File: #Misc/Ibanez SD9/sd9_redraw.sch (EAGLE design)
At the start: 73 parts, among them IC101 RC4558, Q101 2SC1815BL, Q102 1SK44SP, Q103 2SC1815BL, Q104 2SK44SP, Q105 2SC1815BL, Q106 2SC1815BL, Q107 2SC1815BL

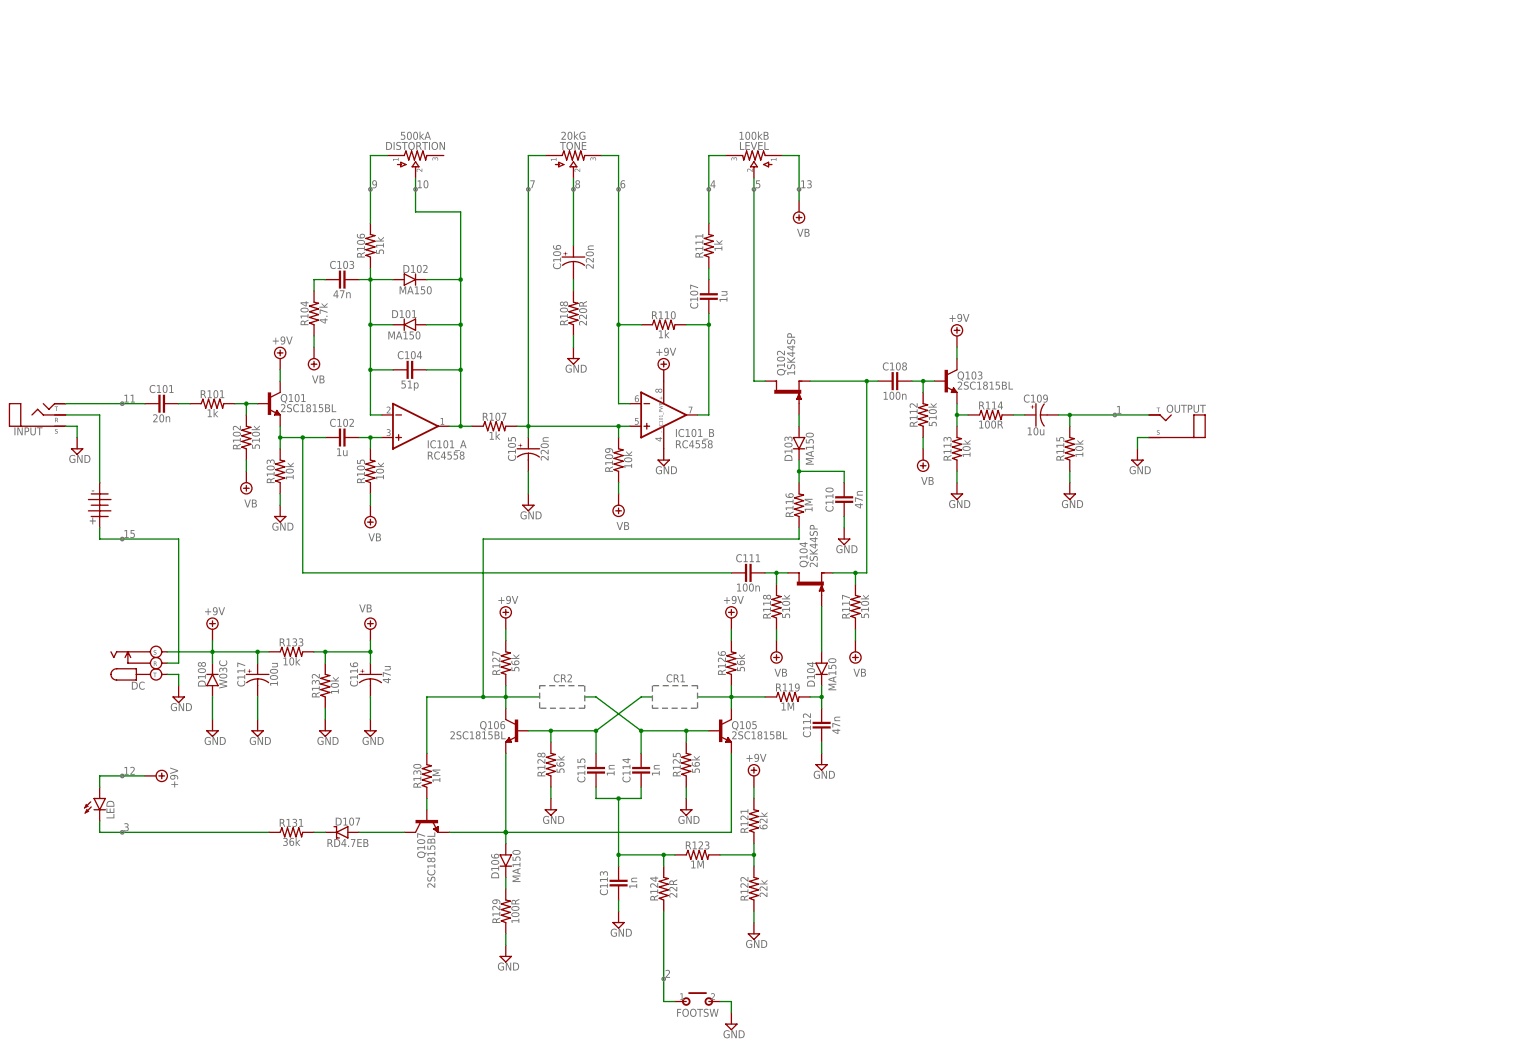
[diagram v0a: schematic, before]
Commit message: 20200325/10:41
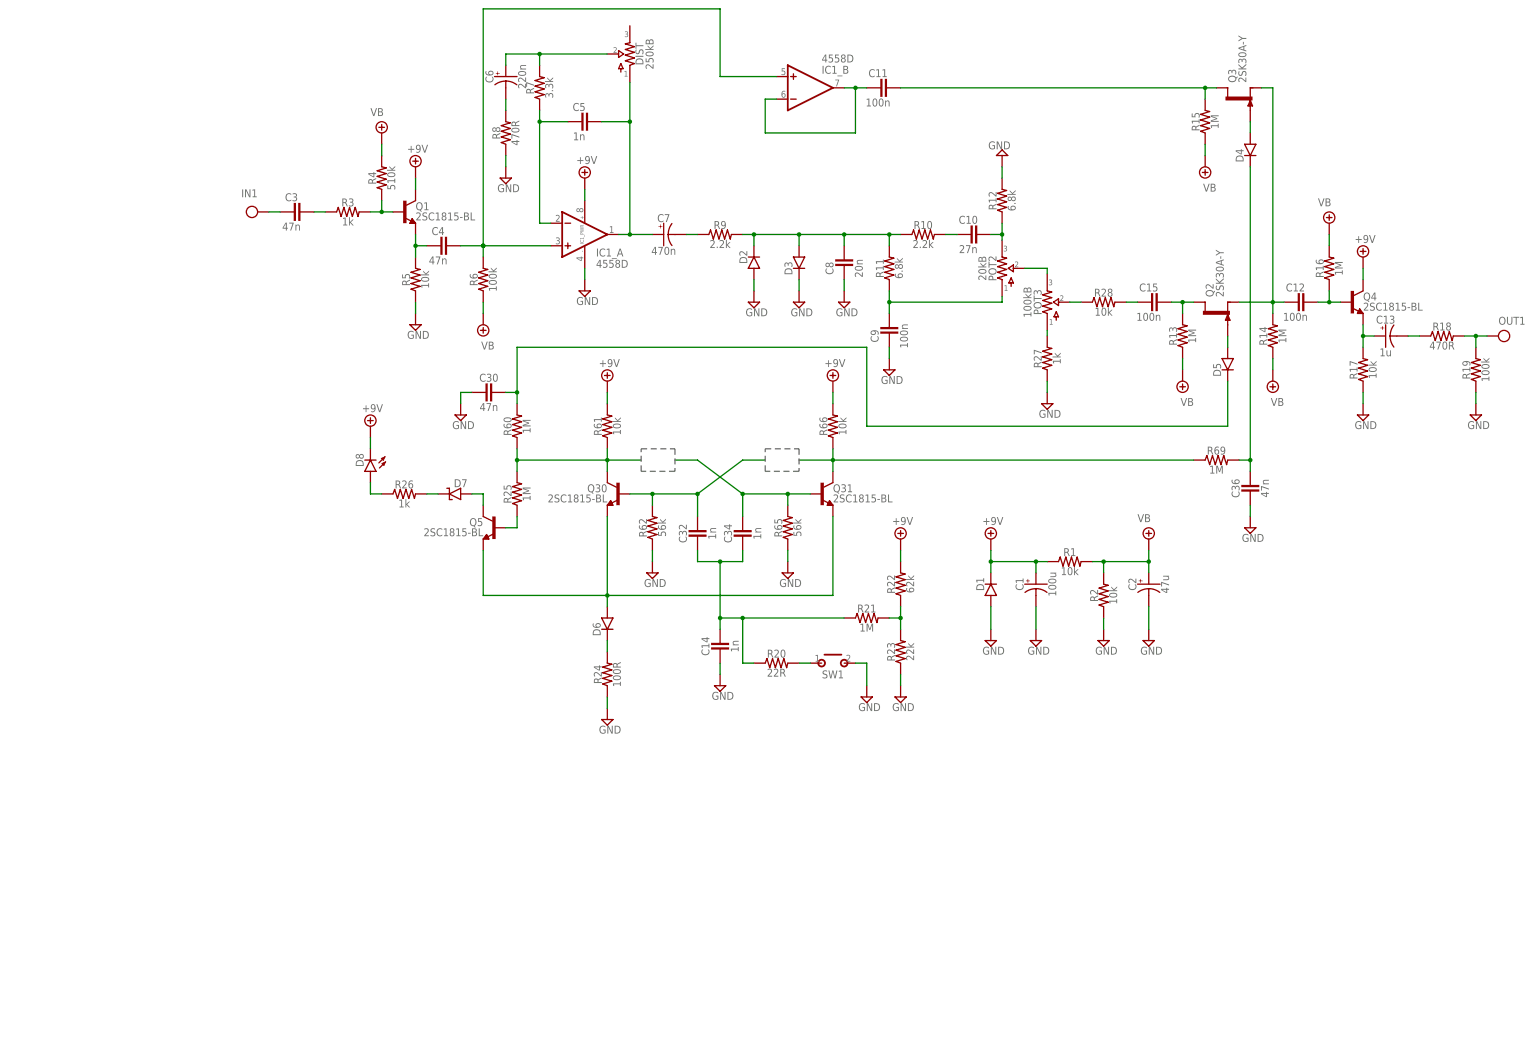
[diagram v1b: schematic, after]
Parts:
- removed BATTERY: BATTERY, pedals-jacks:BATTERY
- removed C101: 20n, pedals-capacitors-film:CER/FILMBOX.1
- removed C102, C107: 1u, pedals-capacitors-film:CER/FILMBOX.1
- removed C103, C110, C112: 47n, pedals-capacitors-film:CER/FILMBOX.1
- removed C104: 51p, pedals-capacitors-film:CER/FILMBOX.1
- removed C105, C106: 220n, pedals-capacitors-elec:0500
- removed C108, C111: 100n, pedals-capacitors-film:CER/FILMBOX.1
- removed C109: 10u, pedals-capacitors-elec:0500
- removed C113, C114, C115: 1n, pedals-capacitors-film:CER/FILMBOX.1
- removed C116: 47u, pedals-capacitors-elec:0500
- removed C117: 100u, pedals-capacitors-elec:0500
- removed D101, D102, D103, D104, D106: MA150, pedals-diodes:DO35.2
- removed D107: RD4.7EB, pedals-diodes:ZENER.2
- removed D108: W03C, pedals-diodes:DO35.2
- removed DC: DCJACK, pedals-jacks:DC_KOBICONN
- removed DISTORTION: 500kA, pedals-potentiometers:POTS16MM
- removed FOOTSW: MOMENTARY, pedals-switches:MOMENTARY
- removed IC101: RC4558, pedals-integrated circuits:DUALTH
- removed INPUT: (no value), pedals-jacks:STEREO3PADS
- removed LED: LED, pedals-diodes:LED
- removed LEVEL: 100kB, pedals-potentiometers:POTS16MM
- removed OUTPUT: (no value), pedals-jacks:MONO
- removed Q101, Q103: 2SC1815BL, pedals-transistors:2N3904
- removed Q102: 1SK44SP, pedals-transistors:2N5457
- removed Q104: 2SK44SP, pedals-transistors:2N5457
- removed Q105, Q106, Q107: 2SC1815BL, pedals-transistors:2SC828A
- removed R101, R107, R110, R111: 1k, pedals-resistors:R_.3B
- removed R102, R112, R117, R118: 510k, pedals-resistors:R_.3B
- removed R103, R105, R109, R113, R115, R132, R133: 10k, pedals-resistors:R_.3B
- removed R104: 4.7k, pedals-resistors:R_.3B
- removed R106: 51k, pedals-resistors:R_.3B
- removed R108: 220R, pedals-resistors:R_.3B
- removed R114, R129: 100R, pedals-resistors:R_.3B
- removed R116, R119, R123, R130: 1M, pedals-resistors:R_.3B
- removed R121: 62k, pedals-resistors:R_.3B
- removed R122: 22k, pedals-resistors:R_.3B
- removed R124: 22R, pedals-resistors:R_.3B
- removed R125, R126, R127, R128: 56k, pedals-resistors:R_.3B
- removed R131: 36k, pedals-resistors:R_.3B
- removed TONE: 20kG, pedals-potentiometers:POTS16MM
- added C1: 100u, pedals-capacitors-elec:0500
- added C10: 27n, pedals-capacitors-film:CER/FILMBOX.1
- added C11, C12, C15, C9: 100n, pedals-capacitors-film:CER/FILMBOX.1
- added C13: 1u, pedals-capacitors-elec:0500
- added C14, C32, C34, C5: 1n, pedals-capacitors-film:CER/FILMBOX.1
- added C2: 47u, pedals-capacitors-elec:0500
- added C3, C30, C36, C4: 47n, pedals-capacitors-film:CER/FILMBOX.1
- added C6: 220n, pedals-capacitors-elec:0500
- added C7: 470n, pedals-capacitors-elec:0500
- added C8: 20n, pedals-capacitors-film:CER/FILMBOX.1
- added D1, D2, D3, D4, D5, D6: (no value), pedals-diodes:DO41.2
- added D7: (no value), pedals-diodes:ZENER.2
- added D8: LED, pedals-diodes:LED
- added DIST: 250kB, pedals-potentiometers:POTS16MM
- added IC1: 4558D, pedals-integrated circuits:DUALTH
- added POT2: 20kB, pedals-potentiometers:POTS16MM
- added POT3: 100kB, pedals-potentiometers:POTS16MM
- added Q1, Q4: 2SC1815-BL, pedals-transistors:2N3904
- added Q2, Q3: 2SK30A-Y, pedals-transistors:2SK170
- added Q30, Q31, Q5: 2SC1815-BL, pedals-transistors:2SC828A
- added R1, R17, R2, R28, R5, R61, R66: 10k, pedals-resistors:R_.3B
- added R10, R9: 2.2k, pedals-resistors:R_.3B
- added R11, R12: 6.8k, pedals-resistors:R_.3B
- added R13, R14, R15, R16, R21, R25, R60, R69: 1M, pedals-resistors:R_.3B
- added R18, R8: 470R, pedals-resistors:R_.3B
- added R19, R6: 100k, pedals-resistors:R_.3B
- added R20: 22R, pedals-resistors:R_.3B
- added R22: 62k, pedals-resistors:R_.3B
- added R23: 22k, pedals-resistors:R_.3B
- added R24: 100R, pedals-resistors:R_.3B
- added R26, R27, R3: 1k, pedals-resistors:R_.3B
- added R4: 510k, pedals-resistors:R_.3B
- added R62, R65: 56k, pedals-resistors:R_.3B
- added R7: 3.3k, pedals-resistors:R_.3B
- added SW1: MOMENTARY, pedals-switches:MOMENTARY
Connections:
- removed net N$1: C101.2, INPUT.T
- removed net N$23: C108.1, Q103.B, R112.2
- removed net N$42: D107.A, Q107.C
- new net IN: C3.2
- new net N$62: C36.1, D4.C, R69.2
- new net N$72: C30.1, D5.C, R60.2
- new net OUT: R18.2, R19.2
- net +9V: now also C1.+, D1.C, D8.C, IC1_PWR.V+, Q1.C, Q4.C, R1.1, R22.2, R61.2, R66.2; no longer C117.+, D108.C, DC.S, IC101_PWR.V+, LED.A, Q101.C, Q103.C, R121.2, R126.2, R127.2, R133.1
- net GND: now also C1.-, C14.2, C2.-, C30.2, C36.2, C8.2, C9.2, D1.A, D2.A, D3.C, IC1_PWR.V-, R12.2, R17.1, R19.1, R2.1, R23.1, R24.1, R27.1, R5.1, R62.1, R65.1, R8.1, SW1.S; no longer C105.-, C110.2, C112.2, C113.2, C116.-, C117.-, D108.A, DC.T, FOOTSW.S, IC101_PWR.V-, INPUT.S, OUTPUT.SLEEVE, R103.1, R108.1, R113.1, R115.1, R122.1, R125.1, R128.1, R129.1, R132.1
- net N$10: now also C7.-, R9.1; no longer C105.+, IC101_B.+IN, R107.2, R109.2, TONE.1
- net N$11: now also C8.1, D2.C, D3.A, R10.1, R11.2, R9.2; no longer IC101_B.-IN, R110.1, TONE.3
- net N$12: now also POT2.2, POT3.3; no longer C107.2, IC101_B.OUT, R110.2
- net N$13: now also C10.2, R10.2; no longer C107.1, R111.1
- net N$14: now also C10.1, POT2.3, R12.1; no longer C106.+, TONE.2
- net N$15: now also C9.1, POT2.1, R11.1; no longer C106.-, R108.2
- net N$16: now also C11.2, IC1_B.-IN, IC1_B.OUT; no longer LEVEL.3, R111.2
- net N$17: now also C11.1, Q3.D, R15.2; no longer LEVEL.2, Q102.D
- net N$18: now also C12.1, Q4.B, R16.1; no longer C108.2, Q102.S, Q104.S, R117.2
- net N$19: now also C12.2, Q2.S, Q3.S, R14.2; no longer D103.A, Q102.G
- net N$2: now also C3.1, R3.1; no longer BATTERY.P$2, INPUT.R
- net N$20: now also C15.1, Q2.D, R13.2; no longer C110.1, D103.C, R116.2
- net N$21: now also C13.+, Q4.E, R17.2; no longer D104.A, Q104.G
- net N$22: now also C13.-, R18.1; no longer C112.1, D104.C, R119.2
- net N$24: now also R20.2, SW1.P; no longer Q103.E, R113.2, R114.1
- net N$25: now also D4.A, Q3.G; no longer C109.+, R114.2
- net N$26: now also D5.A, Q2.G; no longer C109.-, OUTPUT.TIP, R115.2
- net N$27: now also D6.A, Q30.E, Q31.E, Q5.E; no longer C111.1, Q104.D, R118.2
- net N$28: now also Q30.C, R25.2, R60.1, R61.1; no longer BATTERY.P$1, DC.R
- net N$29: now also Q5.B, R25.1; no longer Q106.C, R116.1, R127.1, R130.2
- net N$3: now also Q1.B, R3.2, R4.1; no longer Q101.B, R101.2, R102.2
- net N$30: now also D7.A, Q5.C; no longer Q107.B, R130.1
- net N$31: now also Q31.C, R66.1, R69.1; no longer Q105.C, R119.1, R126.1
- net N$32: now also C32.1, Q30.B, R62.2; no longer C115.1, Q106.B, R128.2
- net N$33: now also D7.C, R26.2; no longer C101.1, R101.1
- net N$34: now also C34.1, Q31.B, R65.2; no longer C114.1, Q105.B, R125.2
- net N$35: now also C14.1, C32.2, C34.2, R20.1, R21.1; no longer D106.A, Q105.E, Q106.E, Q107.E
- net N$36: now also D8.A, R26.1; no longer C113.1, C114.2, C115.2, R123.1, R124.2
- net N$37: now also D6.C, R24.2; no longer D106.C, R129.2
- net N$38: now also POT3.1, R27.2; no longer R121.1, R122.2, R123.2
- net N$39: now also R21.2, R22.1, R23.2; no longer FOOTSW.P, R124.1
- net N$4: now also C4.2, Q1.E, R5.2; no longer C102.2, C111.2, Q101.E, R103.2
- net N$40: now also POT3.2, R28.1; no longer LED.C, R131.1
- net N$41: now also C15.2, R28.2; no longer D107.C, R131.2
- net N$5: now also C4.1, IC1_A.+IN, IC1_B.+IN, R6.2; no longer C102.1, IC101_A.+IN, R105.2
- net N$6: now also C5.2, IC1_A.-IN, R7.1; no longer C103.1, C104.2, D101.C, D102.A, IC101_A.-IN, R106.1
- net N$7: now also C5.1, C7.+, DIST.1, IC1_A.OUT; no longer DISTORTION.1, R106.2
- net N$8: now also C6.+, DIST.2, R7.2; no longer C104.1, D101.A, D102.C, DISTORTION.2, IC101_A.OUT, R107.1
- net N$9: now also C6.-, R8.2; no longer C103.2, R104.2
- net VB: now also C2.+, R1.2, R13.1, R14.1, R15.1, R16.2, R2.2, R4.2, R6.1; no longer C116.+, LEVEL.1, R102.1, R104.1, R105.1, R109.1, R112.1, R117.1, R118.1, R132.2, R133.2
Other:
- note removed: "1"
- note removed: "10"
- note removed: "11"
- note removed: "12"
- note removed: "13"
- note removed: "15"
- note removed: "2"
- note removed: "3"
- note removed: "4"
- note removed: "5"
- note removed: "6"
- note removed: "7"
- note removed: "8"
- note removed: "9"
- note removed: "CR1"
- note removed: "CR2"
